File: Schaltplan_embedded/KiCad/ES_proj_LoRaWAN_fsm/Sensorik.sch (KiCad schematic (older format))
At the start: 22 parts

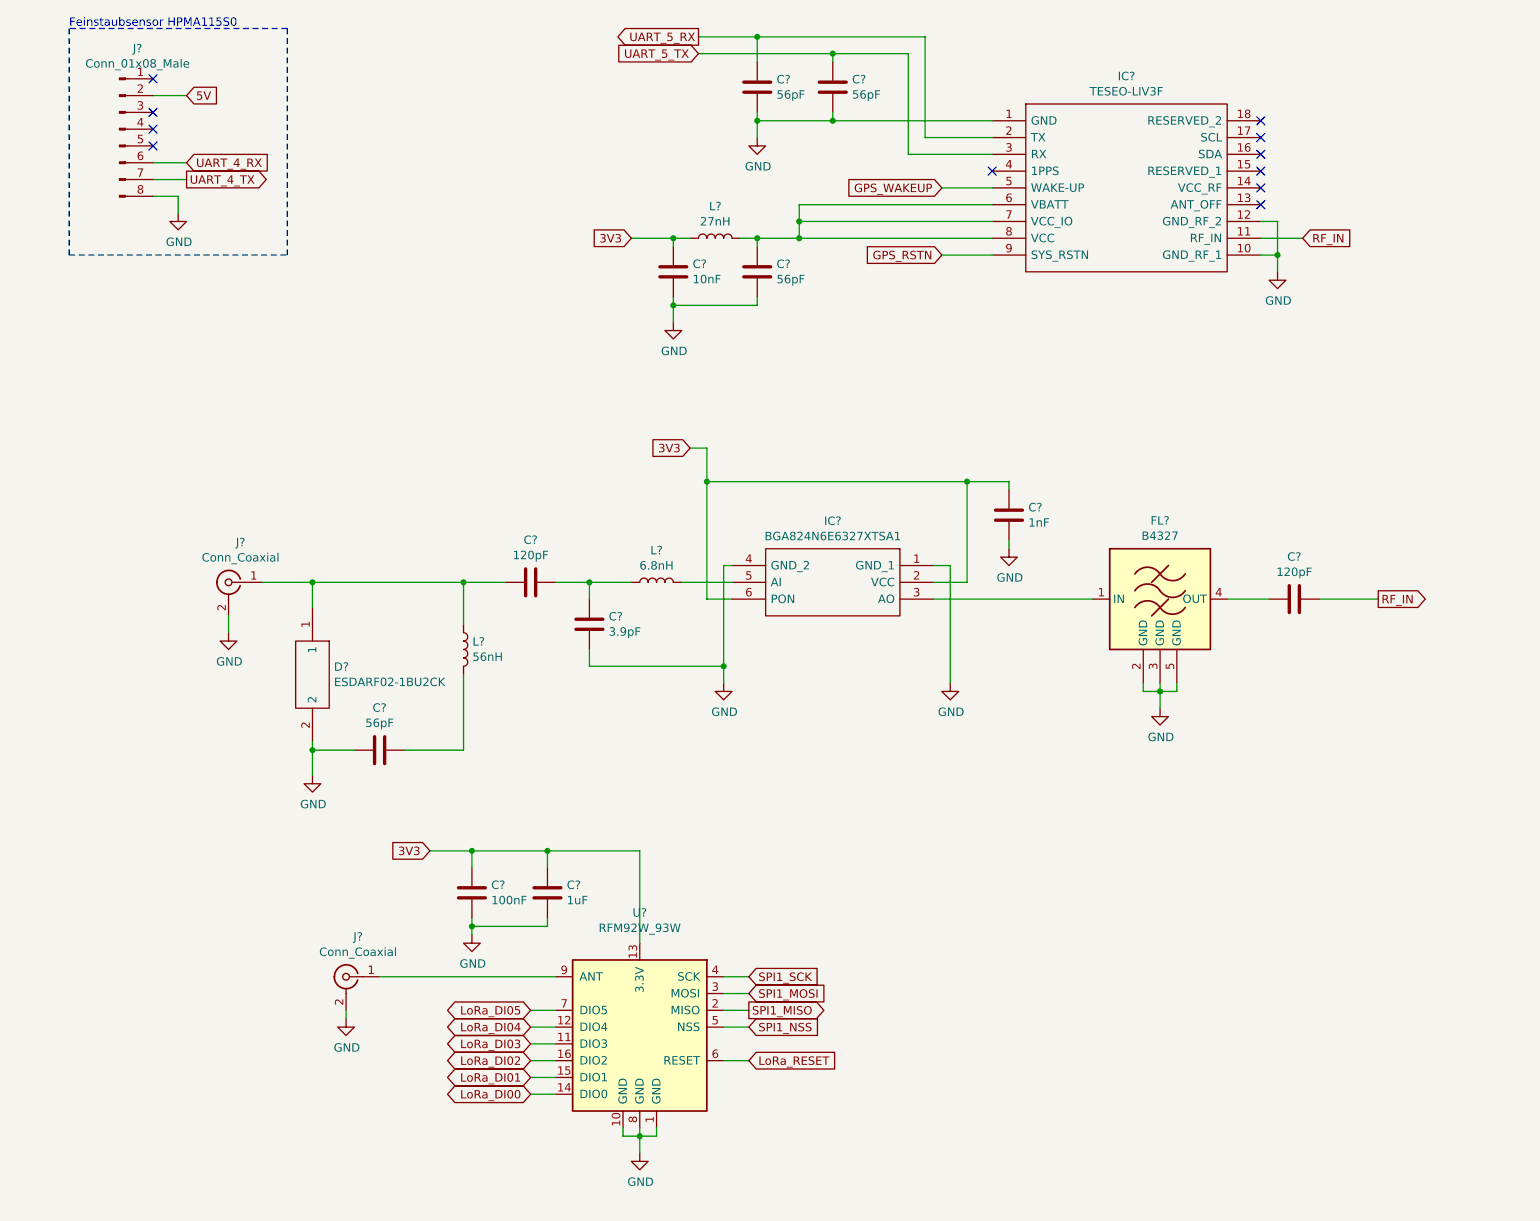
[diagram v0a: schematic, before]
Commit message: Schaltung_Keramik_Antenne
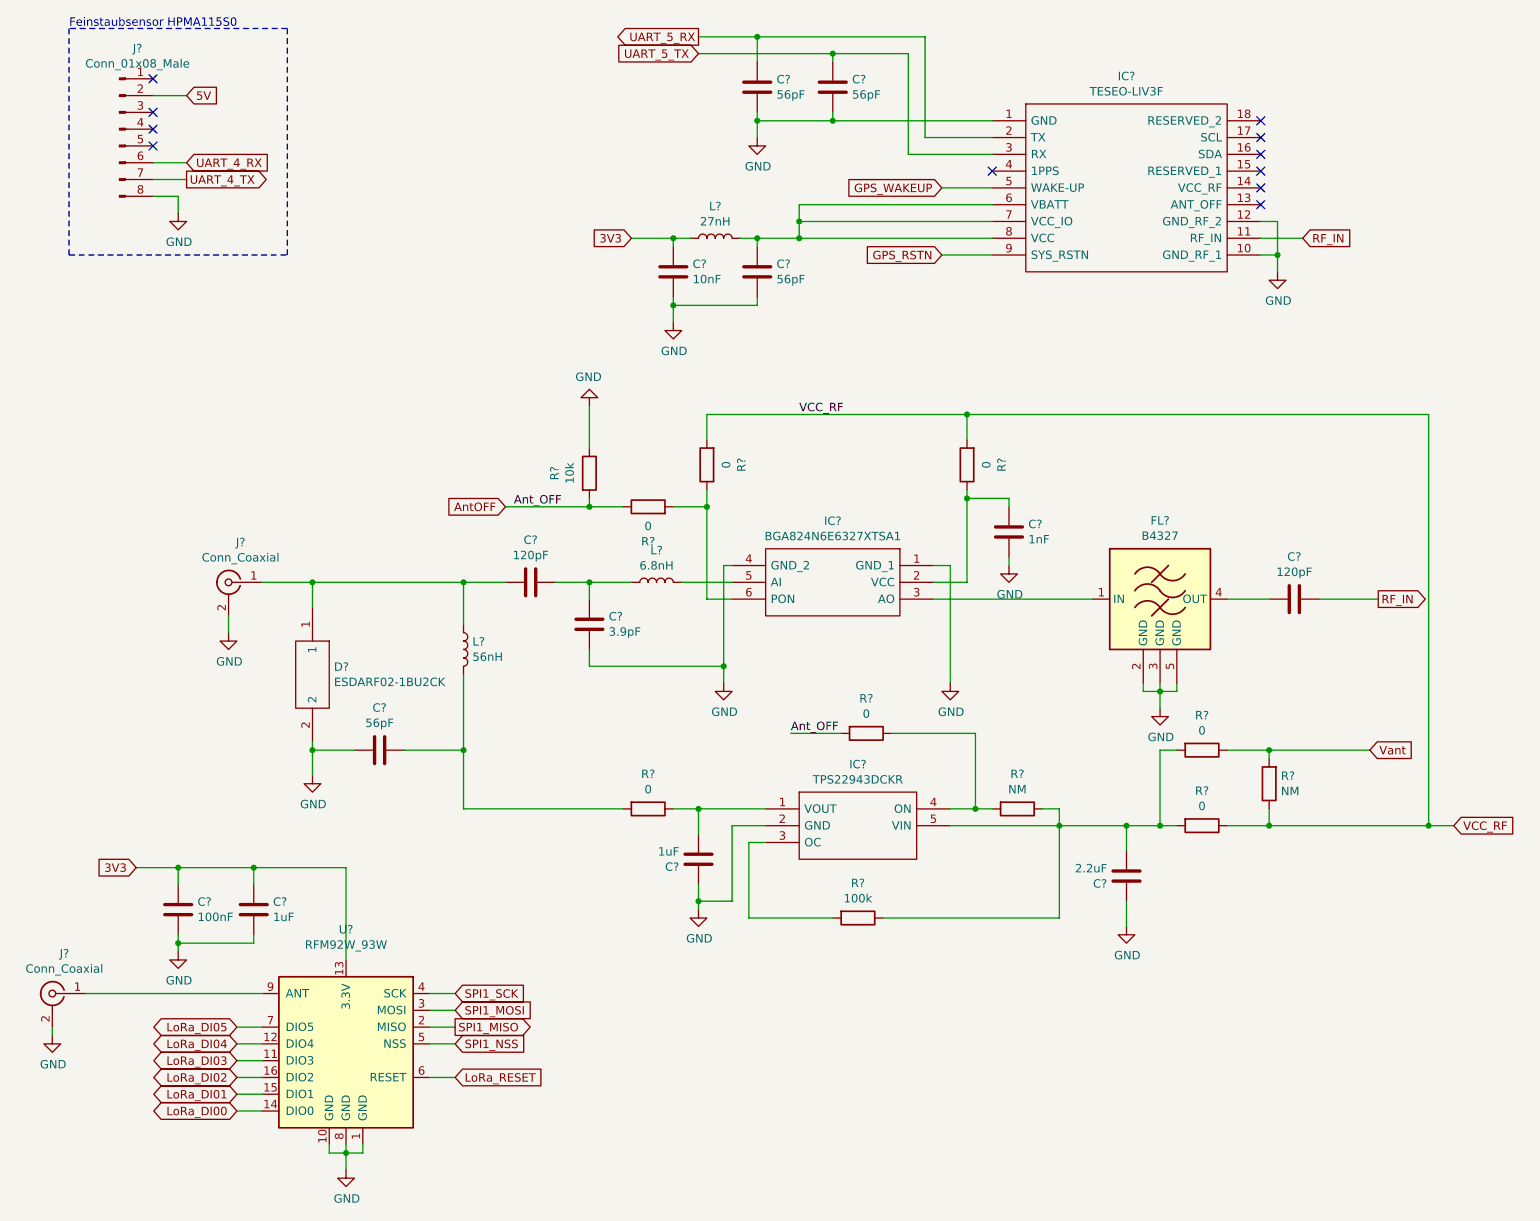
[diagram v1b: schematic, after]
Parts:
- added C?: 1uF, symbol Device:C
- added C?: 2.2uF, symbol Device:C
- added IC?: TPS22943DCKR, SOT65P210X110-5N, symbol SamacSys_Parts:TPS22943DCKR
- added R? (x7): 0, symbol Device:R
- added R? (x2): NM, symbol Device:R
- added R?: 100k, symbol Device:R
- added R?: 10k, symbol Device:R
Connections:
- net 3V3: no longer C?.2, IC?.2 (VCC), IC?.6 (PON)
- net GND: now also C?.2, C?.2, IC?.2 (GND), R?.1
- net at C?.1, L?.2: now also R?.2
- new net: C?.1, IC?.1 (VOUT), R?.1
- new net: C?.1, IC?.5 (VIN), R?.1, R?.1, R?.2, R?.2
- new net: IC?.3 (OC), R?.2
- new net: IC?.4 (ON), R?.1, R?.2
- new net: C?.2, IC?.2 (VCC), R?.1
- new net: IC?.6 (PON), R?.1, R?.2
- new net AntOFF: R?.1, R?.2, R?.2
- new net VCC_RF: R?.1, R?.1, R?.2, R?.2
- new net Vant: R?.1, R?.2
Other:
- moved on the sheet: C?, J?, U?
